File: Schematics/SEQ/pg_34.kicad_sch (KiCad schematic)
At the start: 14 parts, among them U3501 F158, U3502 F158, U3503 F158, U3504 F158, U3505 F158, U3506 F158, U3507 F04, U3508 F240, U3509 F240, U3510 F04, U3511 F258, U3512 F258, U3513 F258, U3514 F258

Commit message: Much work on SEQ
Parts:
- removed U3504, U3505, U3506: F158, symbol r1000:F158
- removed U3508, U3509: F240, symbol r1000:F240
- removed U3510: F04, symbol r1000:F04
- removed U3511, U3512, U3513, U3514: F258, symbol r1000:F258
- U3501: value F158 -> XMUX24; symbol r1000:F158 -> r1000:XMUX24; Location F40 -> x99; Name CODMX0 -> CODMXS
- U3502: value F158 -> XBUF16; symbol r1000:F158 -> r1000:XBUF16; Location F39 -> x99; Name CODMX1 -> CODDR
- U3503: value F158 -> XMUX16; symbol r1000:F158 -> r1000:XMUX16; Location F36 -> x99; Name CODMX2 -> CODMXO
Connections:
- net BRANCH.IND~57: now also U3502.29 (I13)
- net BRANCH.IND~58: now also U3502.31 (I14)
- net BRANCH.IND~59: now also U3502.33 (I15)
- net BRANCH.OFFS~45: now also U3502.5 (I1)
- net BRANCH.OFFS~46: now also U3502.7 (I2)
- net BRANCH.OFFS~47: now also U3502.9 (I3)
- net BRANCH.OFFS~48: now also U3502.11 (I4)
- net BRANCH.OFFS~49: now also U3502.13 (I5)
- net BRANCH.OFFS~50: now also U3502.15 (I6)
- net BRANCH.OFFS~51: now also U3502.17 (I7)
- net BRANCH.OFFS~52: now also U3502.19 (I8)
- net BRANCH.OFFS~53: now also U3502.21 (I9)
- net BRANCH.OFFS~54: now also U3502.23 (I10)
- net BRANCH.OFFS~55: now also U3502.25 (I11)
- net BRANCH.OFFS~56: now also U3502.27 (I12)
- net CODE.IND57: now also U3502.30 (Y13), U3503.48 (Y13)
- net CODE.IND58: now also U3502.32 (Y14), U3503.50 (Y14)
- net CODE.IND59: now also U3502.34 (Y15), U3503.52 (Y15)
- net CODE.OFFS45: now also U3502.6 (Y1), U3503.24 (Y1)
- net CODE.OFFS46: now also U3502.8 (Y2), U3503.26 (Y2)
- net CODE.OFFS47: now also U3502.10 (Y3), U3503.28 (Y3)
- net CODE.OFFS48: now also U3502.12 (Y4), U3503.30 (Y4)
- net CODE.OFFS49: now also U3502.14 (Y5), U3503.32 (Y5)
- net CODE.OFFS50: now also U3502.16 (Y6), U3503.34 (Y6)
- net CODE.OFFS51: now also U3502.18 (Y7), U3503.36 (Y7)
- net CODE.OFFS52: now also U3502.20 (Y8), U3503.38 (Y8)
- net CODE.OFFS53: now also U3502.22 (Y9), U3503.40 (Y9)
- net CODE.OFFS54: now also U3502.24 (Y10), U3503.42 (Y10)
- net CODE.OFFS55: now also U3502.26 (Y11), U3503.44 (Y11)
- net CODE.OFFS56: now also U3502.28 (Y12), U3503.46 (Y12)
- net CODE.SEGN10: now also U3501.34 (Y2); no longer U3501.9 (Y2)
- net CODE.SEGN11: now also U3501.36 (Y3); no longer U3501.12 (Y3)
- net CODE.SEGN12: now also U3501.38 (Y4); no longer U3502.4 (Y0)
- net CODE.SEGN13: now also U3501.40 (Y5); no longer U3502.7 (Y1)
- net CODE.SEGN14: now also U3501.42 (Y6); no longer U3502.9 (Y2)
- net CODE.SEGN15: now also U3501.44 (Y7); no longer U3502.12 (Y3)
- net CODE.SEGN16: now also U3501.46 (Y8); no longer U3503.4 (Y0)
- net CODE.SEGN17: now also U3501.48 (Y9); no longer U3503.7 (Y1)
- net CODE.SEGN18: now also U3501.50 (Y10); no longer U3503.9 (Y2)
- net CODE.SEGN19: now also U3501.52 (Y11); no longer U3503.12 (Y3)
- net CODE.SEGN20: now also U3501.54 (Y12)
- net CODE.SEGN21: now also U3501.56 (Y13)
- net CODE.SEGN22: now also U3501.58 (Y14)
- net CODE.SEGN23: now also U3501.60 (Y15)
- net CODE.SEGN24: now also U3501.62 (Y16)
- net CODE.SEGN25: now also U3501.64 (Y17)
- net CODE.SEGN26: now also U3501.66 (Y18)
- net CODE.SEGN27: now also U3501.68 (Y19)
- net CODE.SEGN28: now also U3501.70 (Y20)
- net CODE.SEGN29: now also U3501.72 (Y21)
- net CODE.SEGN30: now also U3501.74 (Y22)
- net CODE.SEGN31: now also U3501.76 (Y23)
- net CODE.SEGN8: now also U3501.30 (Y0); no longer U3501.4 (Y0)
- net CODE.SEGN9: now also U3501.32 (Y1); no longer U3501.7 (Y1)
- net CODE_SEL.RND0: now also U3501.4 (S), U3503.4 (S); no longer U3501.1 (S), U3502.1 (S), U3503.1 (S)
- net CODE_SEL.RND1: now also U3503.8 (OE)
- net MACRO_PC.IND~57: now also U3503.47 (B13)
- net MACRO_PC.IND~58: now also U3503.49 (B14)
- net MACRO_PC.IND~59: now also U3503.51 (B15)
- net MACRO_PC.OFS~45: now also U3503.23 (B1)
- net MACRO_PC.OFS~46: now also U3503.25 (B2)
- net MACRO_PC.OFS~47: now also U3503.27 (B3)
- net MACRO_PC.OFS~48: now also U3503.29 (B4)
- net MACRO_PC.OFS~49: now also U3503.31 (B5)
- net MACRO_PC.OFS~50: now also U3503.33 (B6)
- net MACRO_PC.OFS~51: now also U3503.35 (B7)
- net MACRO_PC.OFS~52: now also U3503.37 (B8)
- net MACRO_PC.OFS~53: now also U3503.39 (B9)
- net MACRO_PC.OFS~54: now also U3503.41 (B10)
- net MACRO_PC.OFS~55: now also U3503.43 (B11)
- net MACRO_PC.OFS~56: now also U3503.45 (B12)
- net MACRO_PC.SEG~10: now also U3501.33 (B2); no longer U3501.10 (B2)
- net MACRO_PC.SEG~11: now also U3501.35 (B3); no longer U3501.13 (B3)
- net MACRO_PC.SEG~12: now also U3501.37 (B4); no longer U3502.3 (B0)
- net MACRO_PC.SEG~13: now also U3501.39 (B5); no longer U3502.6 (B1)
- net MACRO_PC.SEG~14: now also U3501.41 (B6); no longer U3502.10 (B2)
- net MACRO_PC.SEG~15: now also U3501.43 (B7); no longer U3502.13 (B3)
- net MACRO_PC.SEG~16: now also U3501.45 (B8); no longer U3503.3 (B0)
- net MACRO_PC.SEG~17: now also U3501.47 (B9); no longer U3503.6 (B1)
- net MACRO_PC.SEG~18: now also U3501.49 (B10); no longer U3503.10 (B2)
- net MACRO_PC.SEG~19: now also U3501.51 (B11); no longer U3503.13 (B3)
- net MACRO_PC.SEG~20: now also U3501.53 (B12)
- net MACRO_PC.SEG~21: now also U3501.55 (B13)
- net MACRO_PC.SEG~22: now also U3501.57 (B14)
- net MACRO_PC.SEG~23: now also U3501.59 (B15)
- net MACRO_PC.SEG~24: now also U3501.61 (B16)
- net MACRO_PC.SEG~25: now also U3501.63 (B17)
- net MACRO_PC.SEG~26: now also U3501.65 (B18)
- net MACRO_PC.SEG~27: now also U3501.67 (B19)
- net MACRO_PC.SEG~28: now also U3501.69 (B20)
- net MACRO_PC.SEG~29: now also U3501.71 (B21)
- net MACRO_PC.SEG~30: now also U3501.73 (B22)
- net MACRO_PC.SEG~31: now also U3501.75 (B23)
- net MACRO_PC.SEG~8: now also U3501.29 (B0); no longer U3501.3 (B0)
- net MACRO_PC.SEG~9: now also U3501.31 (B1); no longer U3501.6 (B1)
- net PD: now also U3501.2 (INV), U3501.6 (E), U3501.8 (OE), U3502.1 (INV), U3503.2 (INV), U3503.6 (E); no longer U3501.15 (E), U3502.15 (E), U3503.15 (E)
- net RETRN_PC.IND~57: now also U3503.18 (A13)
- net RETRN_PC.IND~58: now also U3503.19 (A14)
- net RETRN_PC.IND~59: now also U3503.20 (A15)
- net RETRN_PC.OFS~45: now also U3503.3 (A1)
- net RETRN_PC.OFS~46: now also U3503.5 (A2)
- net RETRN_PC.OFS~47: now also U3503.7 (A3)
- net RETRN_PC.OFS~48: now also U3503.9 (A4)
- net RETRN_PC.OFS~49: now also U3503.10 (A5)
- net RETRN_PC.OFS~50: now also U3503.11 (A6)
- net RETRN_PC.OFS~51: now also U3503.12 (A7)
- net RETRN_PC.OFS~52: now also U3503.13 (A8)
- net RETRN_PC.OFS~53: now also U3503.14 (A9)
- net RETRN_PC.OFS~54: now also U3503.15 (A10)
- net RETRN_PC.OFS~55: now also U3503.16 (A11)
- net RETRN_PC.OFS~56: now also U3503.17 (A12)
- net RETRN_PC.SEG~10: now also U3501.5 (A2); no longer U3501.11 (A2)
- net RETRN_PC.SEG~11: now also U3501.7 (A3); no longer U3501.14 (A3)
- net RETRN_PC.SEG~12: now also U3501.9 (A4); no longer U3502.2 (A0)
- net RETRN_PC.SEG~13: now also U3501.10 (A5); no longer U3502.5 (A1)
- net RETRN_PC.SEG~14: now also U3501.11 (A6); no longer U3502.11 (A2)
- net RETRN_PC.SEG~15: now also U3501.12 (A7); no longer U3502.14 (A3)
- net RETRN_PC.SEG~16: now also U3501.13 (A8); no longer U3503.2 (A0)
- net RETRN_PC.SEG~17: now also U3501.14 (A9); no longer U3503.5 (A1)
- net RETRN_PC.SEG~18: now also U3501.15 (A10); no longer U3503.11 (A2)
- net RETRN_PC.SEG~19: now also U3501.16 (A11); no longer U3503.14 (A3)
- net RETRN_PC.SEG~20: now also U3501.17 (A12)
- net RETRN_PC.SEG~21: now also U3501.18 (A13)
- net RETRN_PC.SEG~22: now also U3501.19 (A14)
- net RETRN_PC.SEG~23: now also U3501.20 (A15)
- net RETRN_PC.SEG~24: now also U3501.21 (A16)
- net RETRN_PC.SEG~25: now also U3501.22 (A17)
- net RETRN_PC.SEG~26: now also U3501.23 (A18)
- net RETRN_PC.SEG~27: now also U3501.24 (A19)
- net RETRN_PC.SEG~28: now also U3501.25 (A20)
- net RETRN_PC.SEG~29: now also U3501.26 (A21)
- net RETRN_PC.SEG~30: now also U3501.27 (A22)
- net RETRN_PC.SEG~31: now also U3501.28 (A23)
- net RETRN_PC.SEG~8: now also U3501.1 (A0); no longer U3501.2 (A0)
- net RETRN_PC.SEG~9: now also U3501.3 (A1); no longer U3501.5 (A1)
- net at U3507.2 (Q): now also U3502.2 (OE)
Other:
- moved on the sheet: U3507

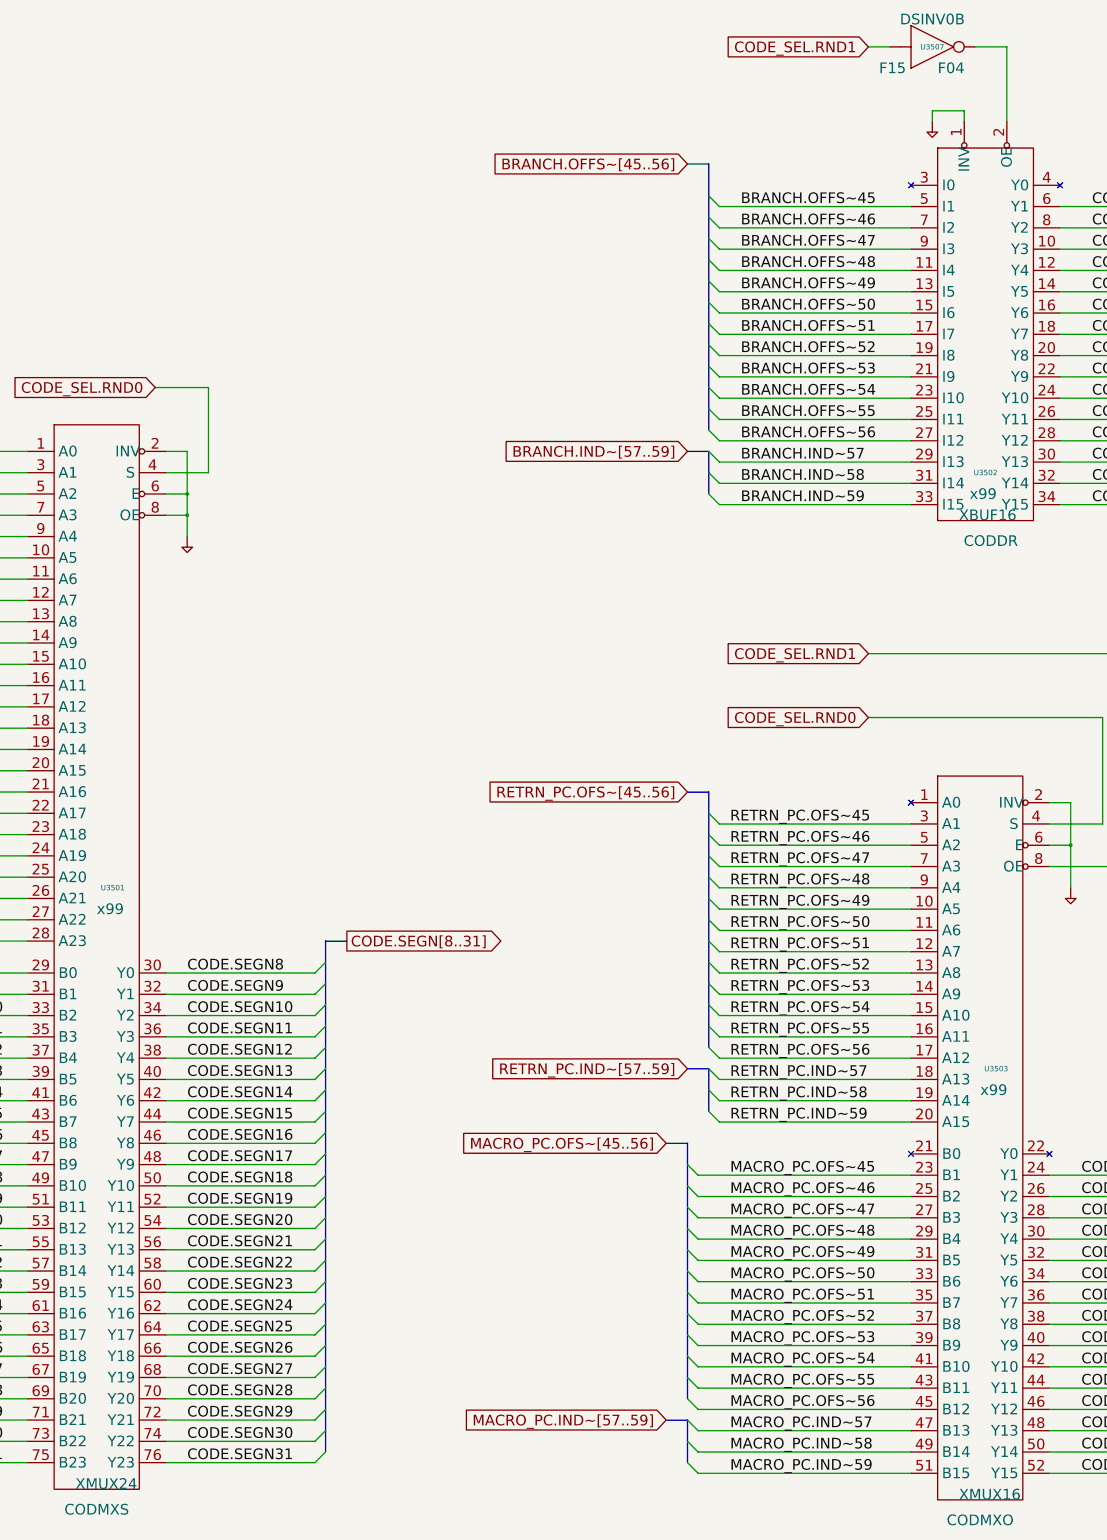
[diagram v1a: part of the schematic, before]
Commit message: KiCad 6
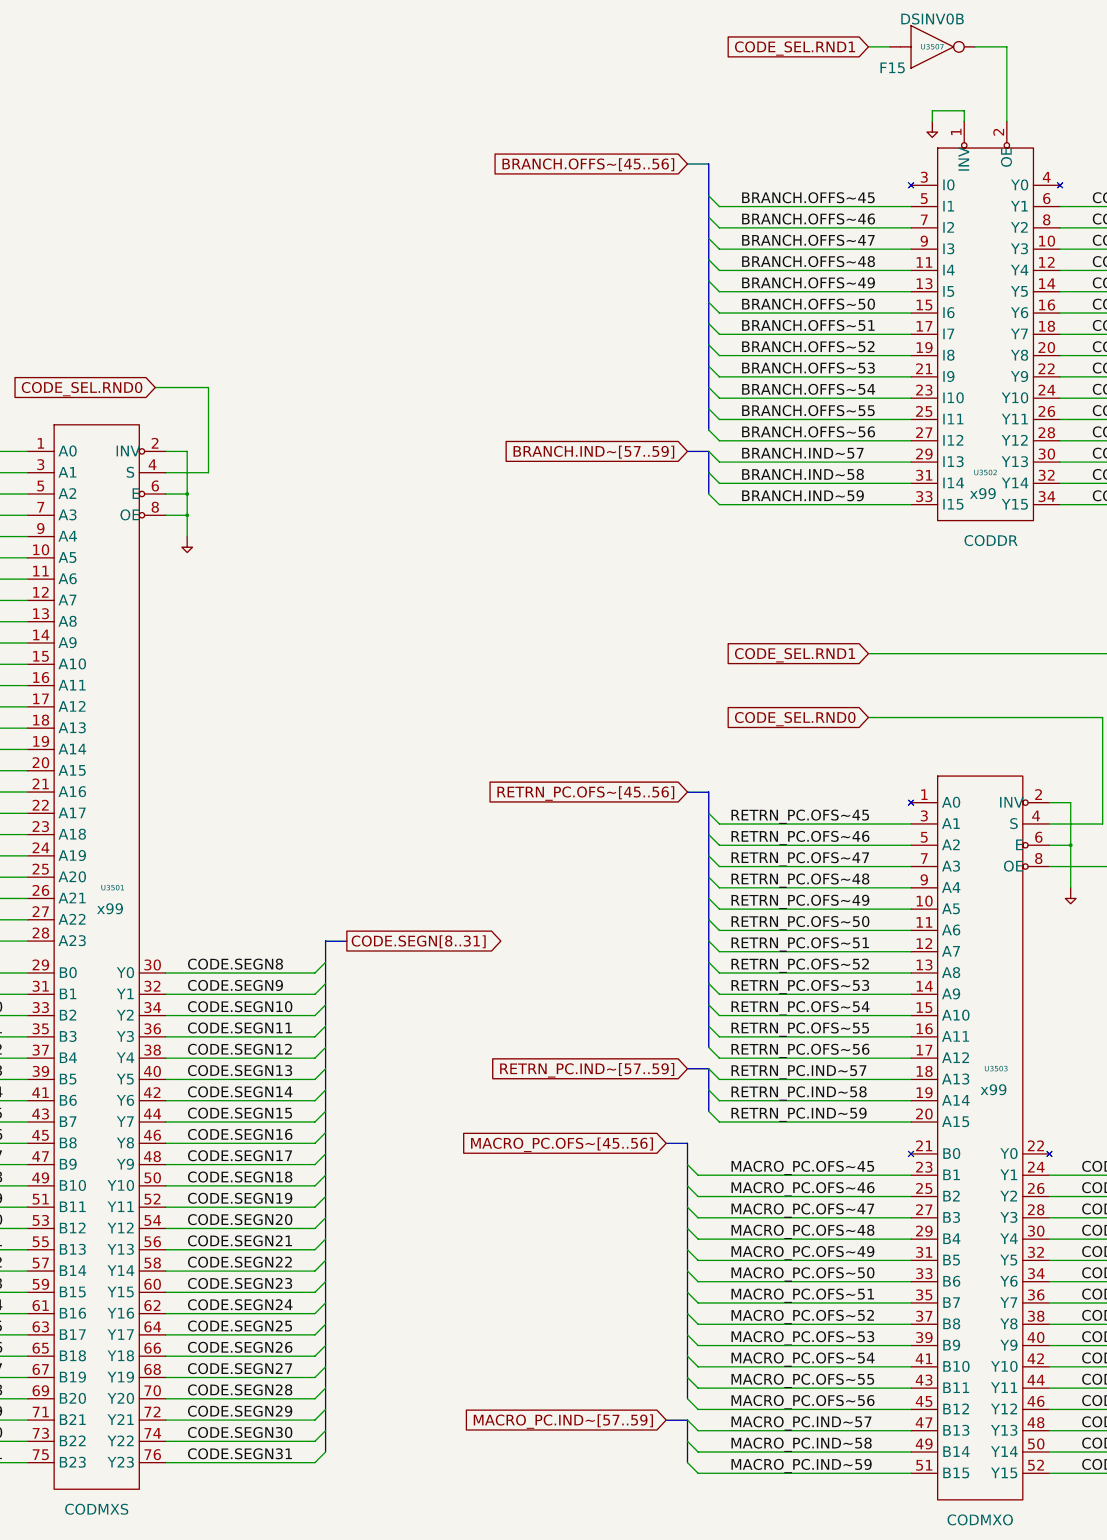
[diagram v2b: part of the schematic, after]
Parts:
- U3501: value XMUX24 -> (none)
- U3502: value XBUF16 -> (none)
- U3503: value XMUX16 -> (none)
- U3507: value F04 -> (none)

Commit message: Recover from KiCad-6 munging
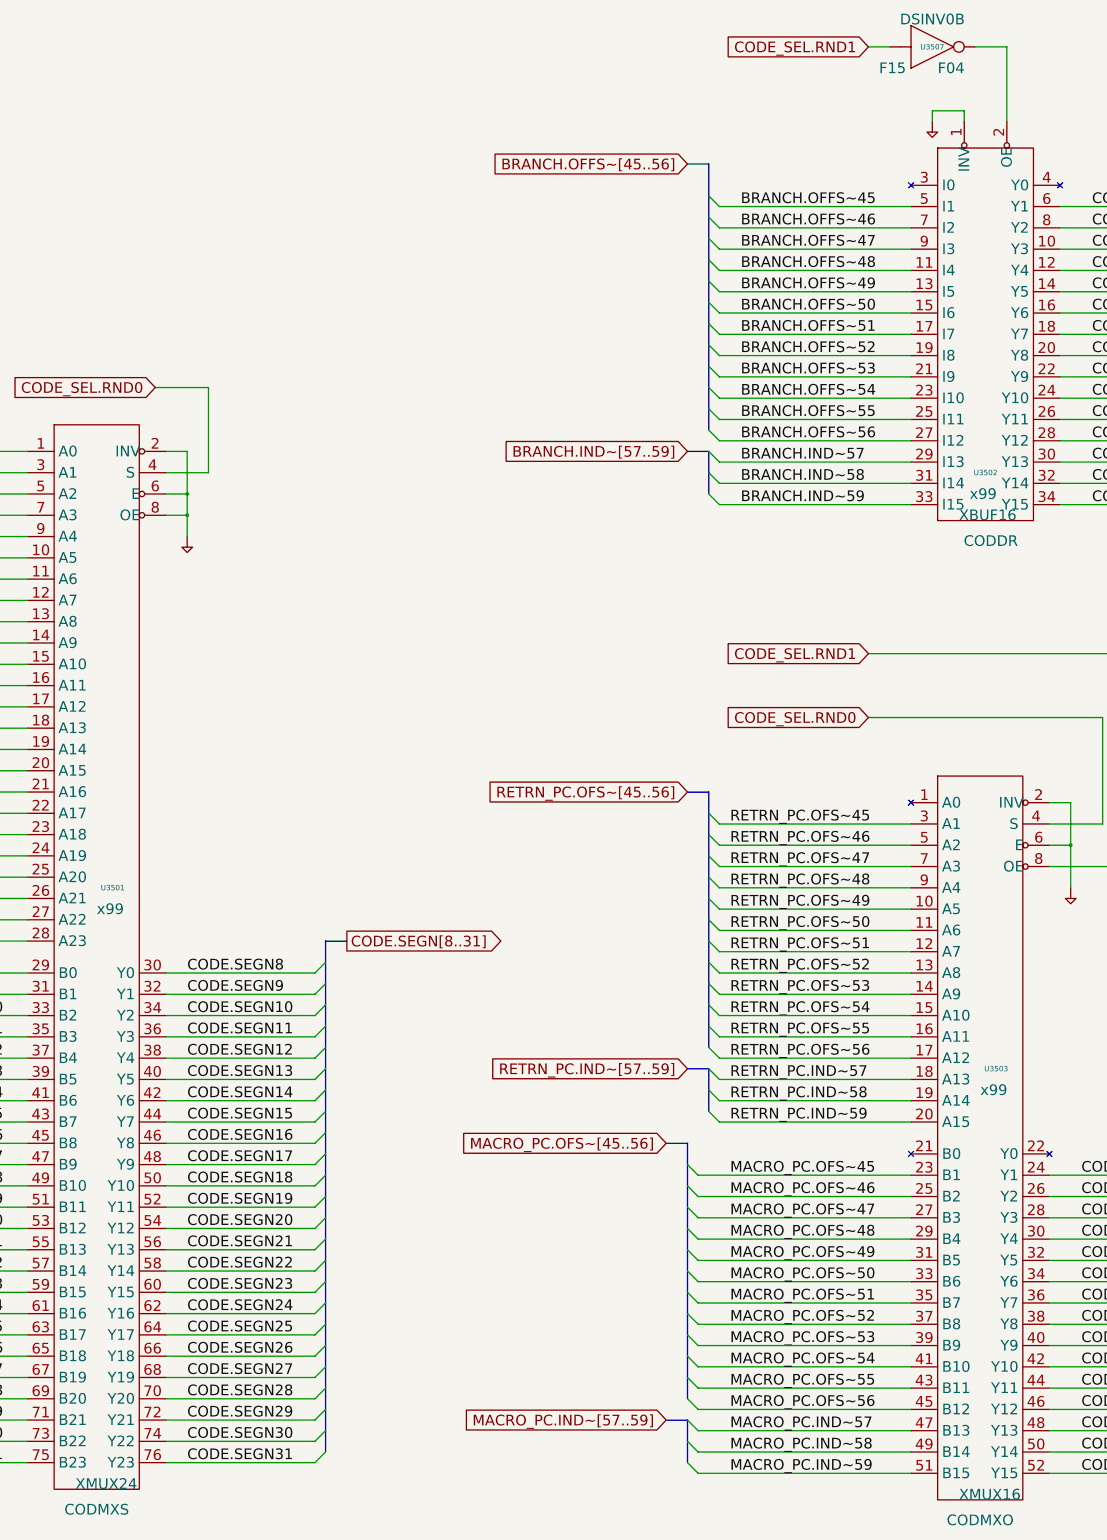
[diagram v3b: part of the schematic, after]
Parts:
- U3501: value (none) -> XMUX24
- U3502: value (none) -> XBUF16
- U3503: value (none) -> XMUX16
- U3507: value (none) -> F04
